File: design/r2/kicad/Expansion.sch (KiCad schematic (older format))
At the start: 22 parts, among them IC1 MC68010P10, J3 Conn_02x32_Odd_Even, J5 PWR

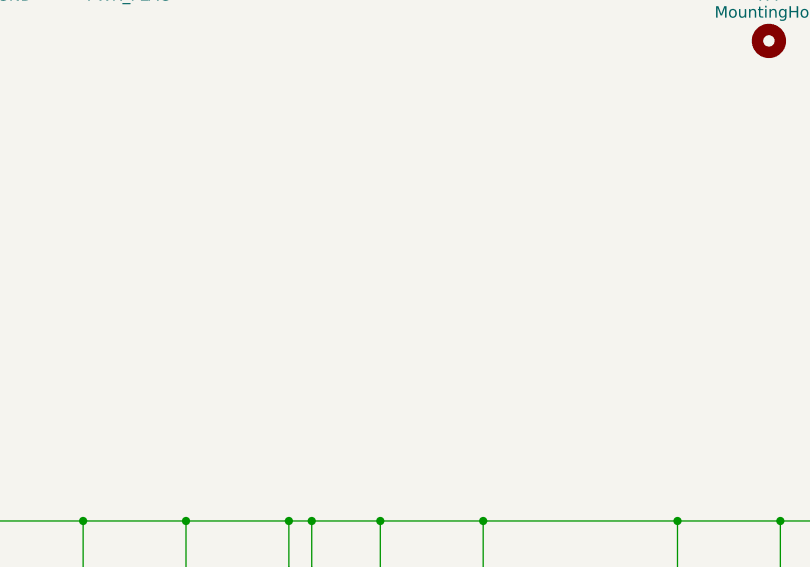
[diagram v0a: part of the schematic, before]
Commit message: Changes requested by @e2k
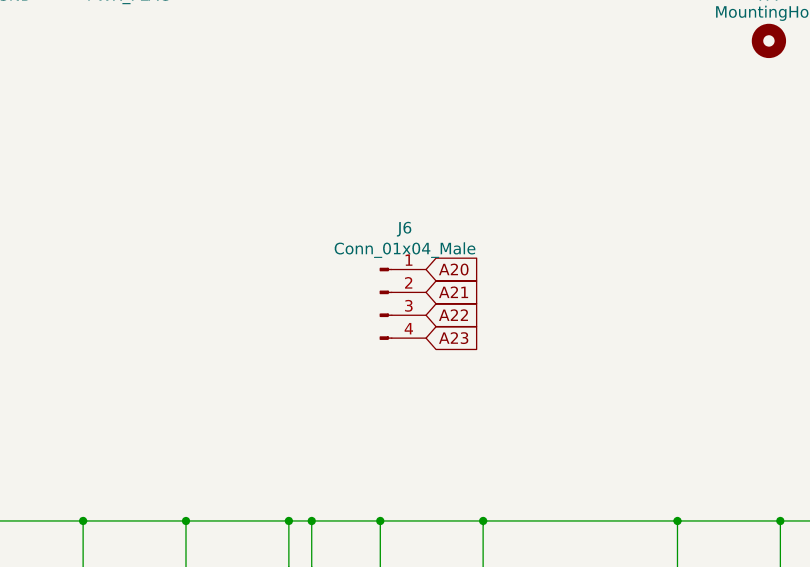
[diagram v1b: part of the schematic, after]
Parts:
- added J6: Conn_01x04_Male, Connector_PinHeader_2.54mm:PinHeader_1x04_P2.54mm_Vertical, symbol Connector:Conn_01x04_Male
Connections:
- net A20: now also J6.1 (Pin_1)
- net A21: now also J6.2 (Pin_2)
- net A22: now also J6.3 (Pin_3)
- net A23: now also J6.4 (Pin_4)
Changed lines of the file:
@@
 Wire Wire Line
 	5500 5750 6300 5750
+$Comp
+L Connector:Conn_01x04_Male J6
+U 1 1 61646A1A
+P 3750 3650
+F 0 "J6" H 3858 3931 50  0000 C CNN
+F 1 "Conn_01x04_Male" H 3858 3840 50  0000 C CNN
+F 2 "Connector_PinHeader_2.54mm:PinHeader_1x04_P2.54mm_Vertical" H 3750 3650 50  0001 C CNN
+F 3 "~" H 3750 3650 50  0001 C CNN
+	1    3750 3650
+	1    0    0    -1
+$EndComp
+Text GLabel 3950 3550 2    50   Input ~ 0
+A20
+Text GLabel 3950 3650 2    50   Input ~ 0
+A21
+Text GLabel 3950 3750 2    50   Input ~ 0
+A22
+Text GLabel 3950 3850 2    50   Input ~ 0
+A23
 $EndSCHEMATC
